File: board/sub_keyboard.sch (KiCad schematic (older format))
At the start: 30 parts, among them SW901 SW_SPST, SW902 SW_SPST, SW903 SW_SPST, SW904 SW_SPST, SW905 SW_SPST, SW906 SW_SPST, SW907 SW_SPST, SW908 SW_SPST, SW909 SW_SPST, SW910 SW_SPST, SW911 SW_SPST, SW912 SW_SPST, SW913 SW_SPST, SW914 SW_SPST, SW915 SW_SPST, SW916 SW_SPST, SW917 SW_SPST, SW918 SW_SPST, SW919 SW_SPST, SW920 SW_SPST, SW921 SW_SPST, SW922 SW_SPST, SW923 SW_SPST, SW924 SW_SPST, SW925 SW_SPST, SW926 SW_SPST, SW927 SW_SPST, SW928 SW_SPST, SW929 SW_SPST, SW930 SW_SPST

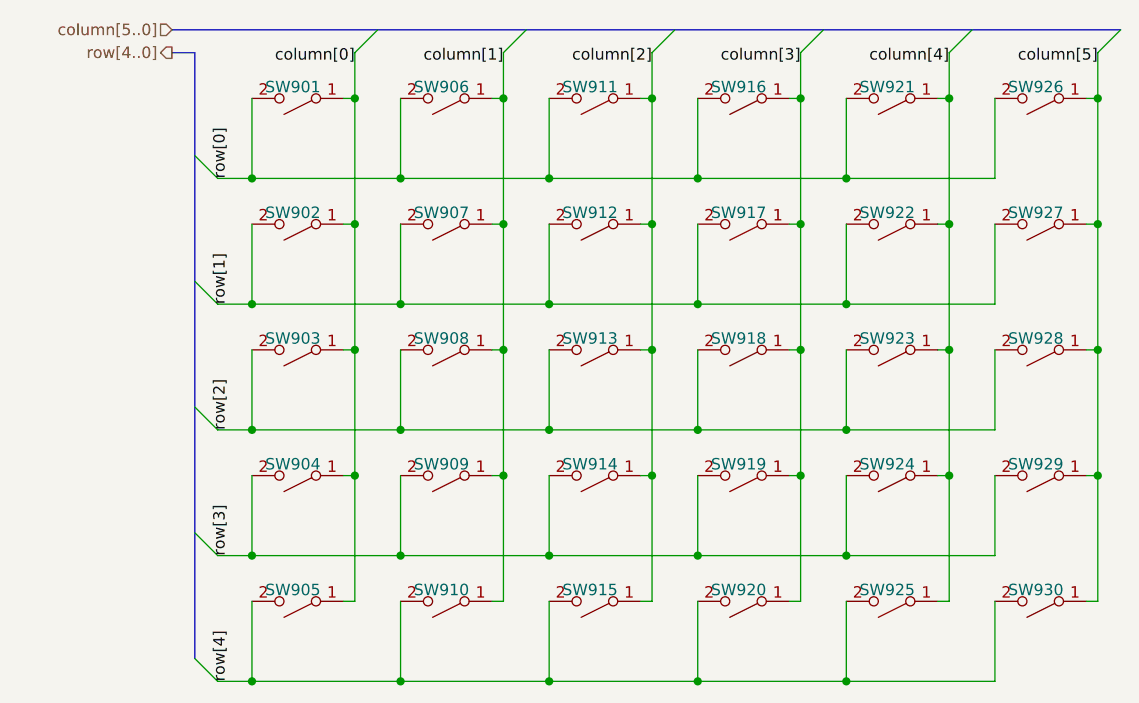
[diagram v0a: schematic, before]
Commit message: Schematics mostly complete
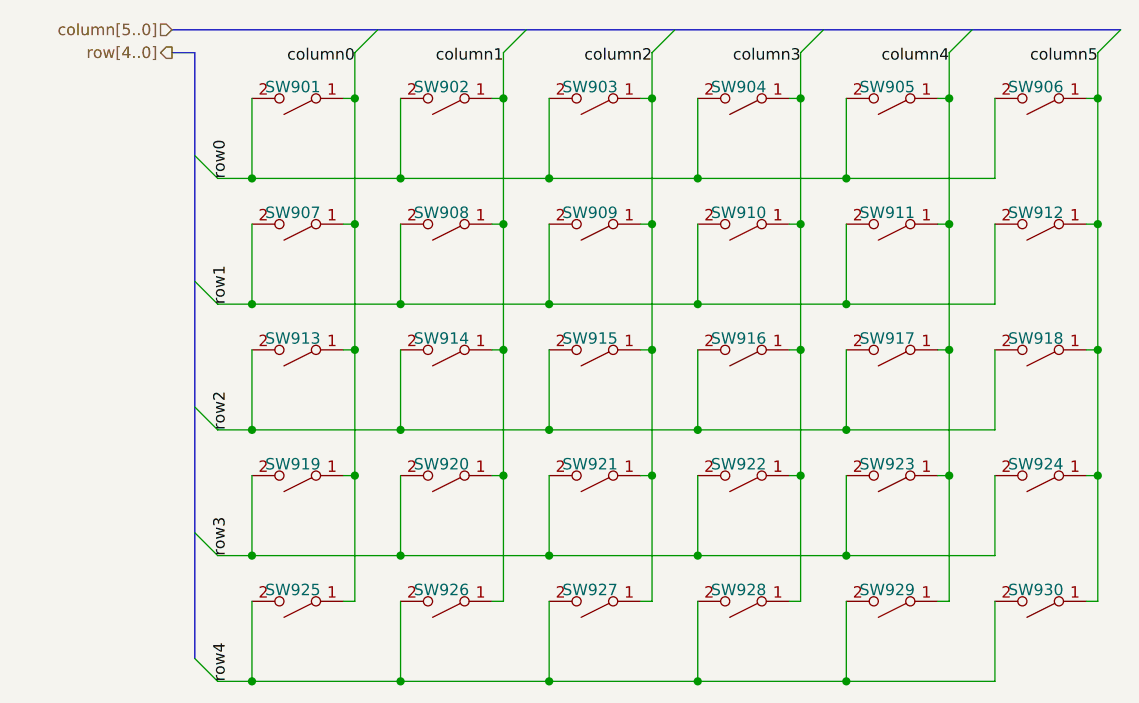
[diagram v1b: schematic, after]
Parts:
- renumbered SW906 to SW902, SW911 to SW903, SW916 to SW904, SW921 to SW905, SW926 to SW906, SW902 to SW907, SW907 to SW908, SW912 to SW909, SW917 to SW910, SW922 to SW911, SW927 to SW912, SW903 to SW913, SW908 to SW914, SW913 to SW915, SW918 to SW916, SW923 to SW917, SW928 to SW918, SW904 to SW919, SW909 to SW920, SW914 to SW921, SW919 to SW922, SW924 to SW923, SW929 to SW924, SW905 to SW925, SW910 to SW926, SW915 to SW927, SW920 to SW928, SW925 to SW929
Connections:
- net column[0] renamed column0
- net column[1] renamed column1
- net column[2] renamed column2
- net column[3] renamed column3
- net column[4] renamed column4
- net column[5] renamed column5
- net row[0] renamed row0
- net row[1] renamed row1
- net row[2] renamed row2
- net row[3] renamed row3
- net row[4] renamed row4
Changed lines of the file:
@@
 $EndComp
 $Comp
-L Switch:SW_SPST SW906
+L Switch:SW_SPST SW902
 U 1 1 5A9F6D51
 P 5250 2500
-F 0 "SW906" H 5150 2450 50  0000 L CNN
+F 0 "SW902" H 5150 2450 50  0000 L CNN
 F 1 "SW_SPST" H 5100 2350 50  0001 L CNN
 F 2 "" H 5250 2500 50  0001 C CNN
@@
 $EndComp
 $Comp
-L Switch:SW_SPST SW911
+L Switch:SW_SPST SW903
 U 1 1 5A9F724F
 P 5900 2500
-F 0 "SW911" H 5800 2450 50  0000 L CNN
+F 0 "SW903" H 5800 2450 50  0000 L CNN
 F 1 "SW_SPST" H 5750 2350 50  0001 L CNN
 F 2 "" H 5900 2500 50  0001 C CNN
@@
 $EndComp
 $Comp
-L Switch:SW_SPST SW916
+L Switch:SW_SPST SW904
 U 1 1 5A9F725B
 P 6550 2500
-F 0 "SW916" H 6450 2450 50  0000 L CNN
+F 0 "SW904" H 6450 2450 50  0000 L CNN
 F 1 "SW_SPST" H 6400 2350 50  0001 L CNN
 F 2 "" H 6550 2500 50  0001 C CNN
@@
 $EndComp
 $Comp
-L Switch:SW_SPST SW921
+L Switch:SW_SPST SW905
 U 1 1 5A9F738F
 P 7200 2500
-F 0 "SW921" H 7100 2450 50  0000 L CNN
+F 0 "SW905" H 7100 2450 50  0000 L CNN
 F 1 "SW_SPST" H 7050 2350 50  0001 L CNN
 F 2 "" H 7200 2500 50  0001 C CNN
@@
 $EndComp
 $Comp
-L Switch:SW_SPST SW926
+L Switch:SW_SPST SW906
 U 1 1 5A9F739B
 P 7850 2500
-F 0 "SW926" H 7750 2450 50  0000 L CNN
+F 0 "SW906" H 7750 2450 50  0000 L CNN
 F 1 "SW_SPST" H 7700 2350 50  0001 L CNN
 F 2 "" H 7850 2500 50  0001 C CNN
@@
 $EndComp
 $Comp
-L Switch:SW_SPST SW902
+L Switch:SW_SPST SW907
 U 1 1 5A9F7527
 P 4600 3050
-F 0 "SW902" H 4500 3000 50  0000 L CNN
+F 0 "SW907" H 4500 3000 50  0000 L CNN
 F 1 "SW_SPST" H 4450 2900 50  0001 L CNN
 F 2 "" H 4600 3050 50  0001 C CNN
@@
 $EndComp
 $Comp
-L Switch:SW_SPST SW907
+L Switch:SW_SPST SW908
 U 1 1 5A9F7533
 P 5250 3050
-F 0 "SW907" H 5150 3000 50  0000 L CNN
+F 0 "SW908" H 5150 3000 50  0000 L CNN
 F 1 "SW_SPST" H 5100 2900 50  0001 L CNN
 F 2 "" H 5250 3050 50  0001 C CNN
@@
 $EndComp
 $Comp
-L Switch:SW_SPST SW912
+L Switch:SW_SPST SW909
 U 1 1 5A9F753F
 P 5900 3050
-F 0 "SW912" H 5800 3000 50  0000 L CNN
+F 0 "SW909" H 5800 3000 50  0000 L CNN
 F 1 "SW_SPST" H 5750 2900 50  0001 L CNN
 F 2 "" H 5900 3050 50  0001 C CNN
@@
 $EndComp
 $Comp
-L Switch:SW_SPST SW917
+L Switch:SW_SPST SW910
 U 1 1 5A9F754B
 P 6550 3050
-F 0 "SW917" H 6450 3000 50  0000 L CNN
+F 0 "SW910" H 6450 3000 50  0000 L CNN
 F 1 "SW_SPST" H 6400 2900 50  0001 L CNN
 F 2 "" H 6550 3050 50  0001 C CNN
@@
 $EndComp
 $Comp
-L Switch:SW_SPST SW922
+L Switch:SW_SPST SW911
 U 1 1 5A9F7557
 P 7200 3050
-F 0 "SW922" H 7100 3000 50  0000 L CNN
+F 0 "SW911" H 7100 3000 50  0000 L CNN
 F 1 "SW_SPST" H 7050 2900 50  0001 L CNN
 F 2 "" H 7200 3050 50  0001 C CNN
@@
 $EndComp
 $Comp
-L Switch:SW_SPST SW927
+L Switch:SW_SPST SW912
 U 1 1 5A9F7563
 P 7850 3050
-F 0 "SW927" H 7750 3000 50  0000 L CNN
+F 0 "SW912" H 7750 3000 50  0000 L CNN
 F 1 "SW_SPST" H 7700 2900 50  0001 L CNN
 F 2 "" H 7850 3050 50  0001 C CNN
@@
 $EndComp
 $Comp
-L Switch:SW_SPST SW903
+L Switch:SW_SPST SW913
 U 1 1 5A9F8C97
 P 4600 3600
-F 0 "SW903" H 4500 3550 50  0000 L CNN
+F 0 "SW913" H 4500 3550 50  0000 L CNN
 F 1 "SW_SPST" H 4450 3450 50  0001 L CNN
 F 2 "" H 4600 3600 50  0001 C CNN
@@
 $EndComp
 $Comp
-L Switch:SW_SPST SW908
+L Switch:SW_SPST SW914
 U 1 1 5A9F8CA3
 P 5250 3600
-F 0 "SW908" H 5150 3550 50  0000 L CNN
+F 0 "SW914" H 5150 3550 50  0000 L CNN
 F 1 "SW_SPST" H 5100 3450 50  0001 L CNN
 F 2 "" H 5250 3600 50  0001 C CNN
@@
 $EndComp
 $Comp
-L Switch:SW_SPST SW913
+L Switch:SW_SPST SW915
 U 1 1 5A9F8CAF
 P 5900 3600
-F 0 "SW913" H 5800 3550 50  0000 L CNN
+F 0 "SW915" H 5800 3550 50  0000 L CNN
 F 1 "SW_SPST" H 5750 3450 50  0001 L CNN
 F 2 "" H 5900 3600 50  0001 C CNN
@@
 $EndComp
 $Comp
-L Switch:SW_SPST SW918
+L Switch:SW_SPST SW916
 U 1 1 5A9F8CBB
 P 6550 3600
-F 0 "SW918" H 6450 3550 50  0000 L CNN
+F 0 "SW916" H 6450 3550 50  0000 L CNN
 F 1 "SW_SPST" H 6400 3450 50  0001 L CNN
 F 2 "" H 6550 3600 50  0001 C CNN
@@
 $EndComp
 $Comp
-L Switch:SW_SPST SW923
+L Switch:SW_SPST SW917
 U 1 1 5A9F8CC7
 P 7200 3600
-F 0 "SW923" H 7100 3550 50  0000 L CNN
+F 0 "SW917" H 7100 3550 50  0000 L CNN
 F 1 "SW_SPST" H 7050 3450 50  0001 L CNN
 F 2 "" H 7200 3600 50  0001 C CNN
@@
 $EndComp
 $Comp
-L Switch:SW_SPST SW928
+L Switch:SW_SPST SW918
 U 1 1 5A9F8CD3
 P 7850 3600
-F 0 "SW928" H 7750 3550 50  0000 L CNN
+F 0 "SW918" H 7750 3550 50  0000 L CNN
 F 1 "SW_SPST" H 7700 3450 50  0001 L CNN
 F 2 "" H 7850 3600 50  0001 C CNN
@@
 $EndComp
 $Comp
-L Switch:SW_SPST SW904
+L Switch:SW_SPST SW919
 U 1 1 5A9F94D7
 P 4600 4150
-F 0 "SW904" H 4500 4100 50  0000 L CNN
+F 0 "SW919" H 4500 4100 50  0000 L CNN
 F 1 "SW_SPST" H 4450 4000 50  0001 L CNN
 F 2 "" H 4600 4150 50  0001 C CNN
@@
 $EndComp
 $Comp
-L Switch:SW_SPST SW909
+L Switch:SW_SPST SW920
 U 1 1 5A9F94E3
 P 5250 4150
-F 0 "SW909" H 5150 4100 50  0000 L CNN
+F 0 "SW920" H 5150 4100 50  0000 L CNN
 F 1 "SW_SPST" H 5100 4000 50  0001 L CNN
 F 2 "" H 5250 4150 50  0001 C CNN
@@
 $EndComp
 $Comp
-L Switch:SW_SPST SW914
+L Switch:SW_SPST SW921
 U 1 1 5A9F94EF
 P 5900 4150
-F 0 "SW914" H 5800 4100 50  0000 L CNN
+F 0 "SW921" H 5800 4100 50  0000 L CNN
 F 1 "SW_SPST" H 5750 4000 50  0001 L CNN
 F 2 "" H 5900 4150 50  0001 C CNN
@@
 $EndComp
 $Comp
-L Switch:SW_SPST SW919
+L Switch:SW_SPST SW922
 U 1 1 5A9F94FB
 P 6550 4150
-F 0 "SW919" H 6450 4100 50  0000 L CNN
+F 0 "SW922" H 6450 4100 50  0000 L CNN
 F 1 "SW_SPST" H 6400 4000 50  0001 L CNN
 F 2 "" H 6550 4150 50  0001 C CNN
@@
 $EndComp
 $Comp
-L Switch:SW_SPST SW924
+L Switch:SW_SPST SW923
 U 1 1 5A9F9507
 P 7200 4150
-F 0 "SW924" H 7100 4100 50  0000 L CNN
+F 0 "SW923" H 7100 4100 50  0000 L CNN
 F 1 "SW_SPST" H 7050 4000 50  0001 L CNN
 F 2 "" H 7200 4150 50  0001 C CNN
@@
 $EndComp
 $Comp
-L Switch:SW_SPST SW929
+L Switch:SW_SPST SW924
 U 1 1 5A9F9513
 P 7850 4150
-F 0 "SW929" H 7750 4100 50  0000 L CNN
+F 0 "SW924" H 7750 4100 50  0000 L CNN
 F 1 "SW_SPST" H 7700 4000 50  0001 L CNN
 F 2 "" H 7850 4150 50  0001 C CNN
@@
 $EndComp
 $Comp
-L Switch:SW_SPST SW905
+L Switch:SW_SPST SW925
 U 1 1 5A9F951F
 P 4600 4700
-F 0 "SW905" H 4500 4650 50  0000 L CNN
+F 0 "SW925" H 4500 4650 50  0000 L CNN
 F 1 "SW_SPST" H 4450 4550 50  0001 L CNN
 F 2 "" H 4600 4700 50  0001 C CNN
@@
 $EndComp
 $Comp
-L Switch:SW_SPST SW910
+L Switch:SW_SPST SW926
 U 1 1 5A9F952B
 P 5250 4700
-F 0 "SW910" H 5150 4650 50  0000 L CNN
+F 0 "SW926" H 5150 4650 50  0000 L CNN
 F 1 "SW_SPST" H 5100 4550 50  0001 L CNN
 F 2 "" H 5250 4700 50  0001 C CNN
@@
 $EndComp
 $Comp
-L Switch:SW_SPST SW915
+L Switch:SW_SPST SW927
 U 1 1 5A9F9537
 P 5900 4700
-F 0 "SW915" H 5800 4650 50  0000 L CNN
+F 0 "SW927" H 5800 4650 50  0000 L CNN
 F 1 "SW_SPST" H 5750 4550 50  0001 L CNN
 F 2 "" H 5900 4700 50  0001 C CNN
@@
 $EndComp
 $Comp
-L Switch:SW_SPST SW920
+L Switch:SW_SPST SW928
 U 1 1 5A9F9543
 P 6550 4700
-F 0 "SW920" H 6450 4650 50  0000 L CNN
+F 0 "SW928" H 6450 4650 50  0000 L CNN
 F 1 "SW_SPST" H 6400 4550 50  0001 L CNN
 F 2 "" H 6550 4700 50  0001 C CNN
@@
 $EndComp
 $Comp
-L Switch:SW_SPST SW925
+L Switch:SW_SPST SW929
 U 1 1 5A9F954F
 P 7200 4700
-F 0 "SW925" H 7100 4650 50  0000 L CNN
+F 0 "SW929" H 7100 4650 50  0000 L CNN
 F 1 "SW_SPST" H 7050 4550 50  0001 L CNN
 F 2 "" H 7200 4700 50  0001 C CNN
@@
 	8100 2300 8200 2200
 Text Label 4850 2350 2    50   ~ 0
-column[0]
+column0
 Text Label 5500 2350 2    50   ~ 0
-column[1]
+column1
 Text Label 6150 2350 2    50   ~ 0
-column[2]
+column2
 Text Label 6800 2350 2    50   ~ 0
-column[3]
+column3
 Text Label 7450 2350 2    50   ~ 0
-column[4]
+column4
 Text Label 8100 2350 2    50   ~ 0
-column[5]
+column5
 Entry Wire Line
 	4150 2750 4250 2850
@@
 	4150 2300 4050 2300
 Text Label 4300 2850 1    50   ~ 0
-row[0]
+row0
 Text Label 4300 3400 1    50   ~ 0
-row[1]
+row1
 Text Label 4300 3950 1    50   ~ 0
-row[2]
+row2
 Text Label 4300 4500 1    50   ~ 0
-row[3]
+row3
 Text Label 4300 5050 1    50   ~ 0
-row[4]
+row4
 Wire Wire Line
 	7650 2500 7650 2850
